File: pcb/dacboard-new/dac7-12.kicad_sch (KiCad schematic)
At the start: 30 parts, among them U22 AD8676xR, U23 AD8676xR, U24 AD8676xR, U25 AD8676xR, U26 AD5791BRUZ, U27 AD5791BRUZ, U28 AD5791BRUZ, U29 AD5791BRUZ, U30 AD8676xR, U31 AD8676xR, U32 AD5791BRUZ, U33 AD5791BRUZ

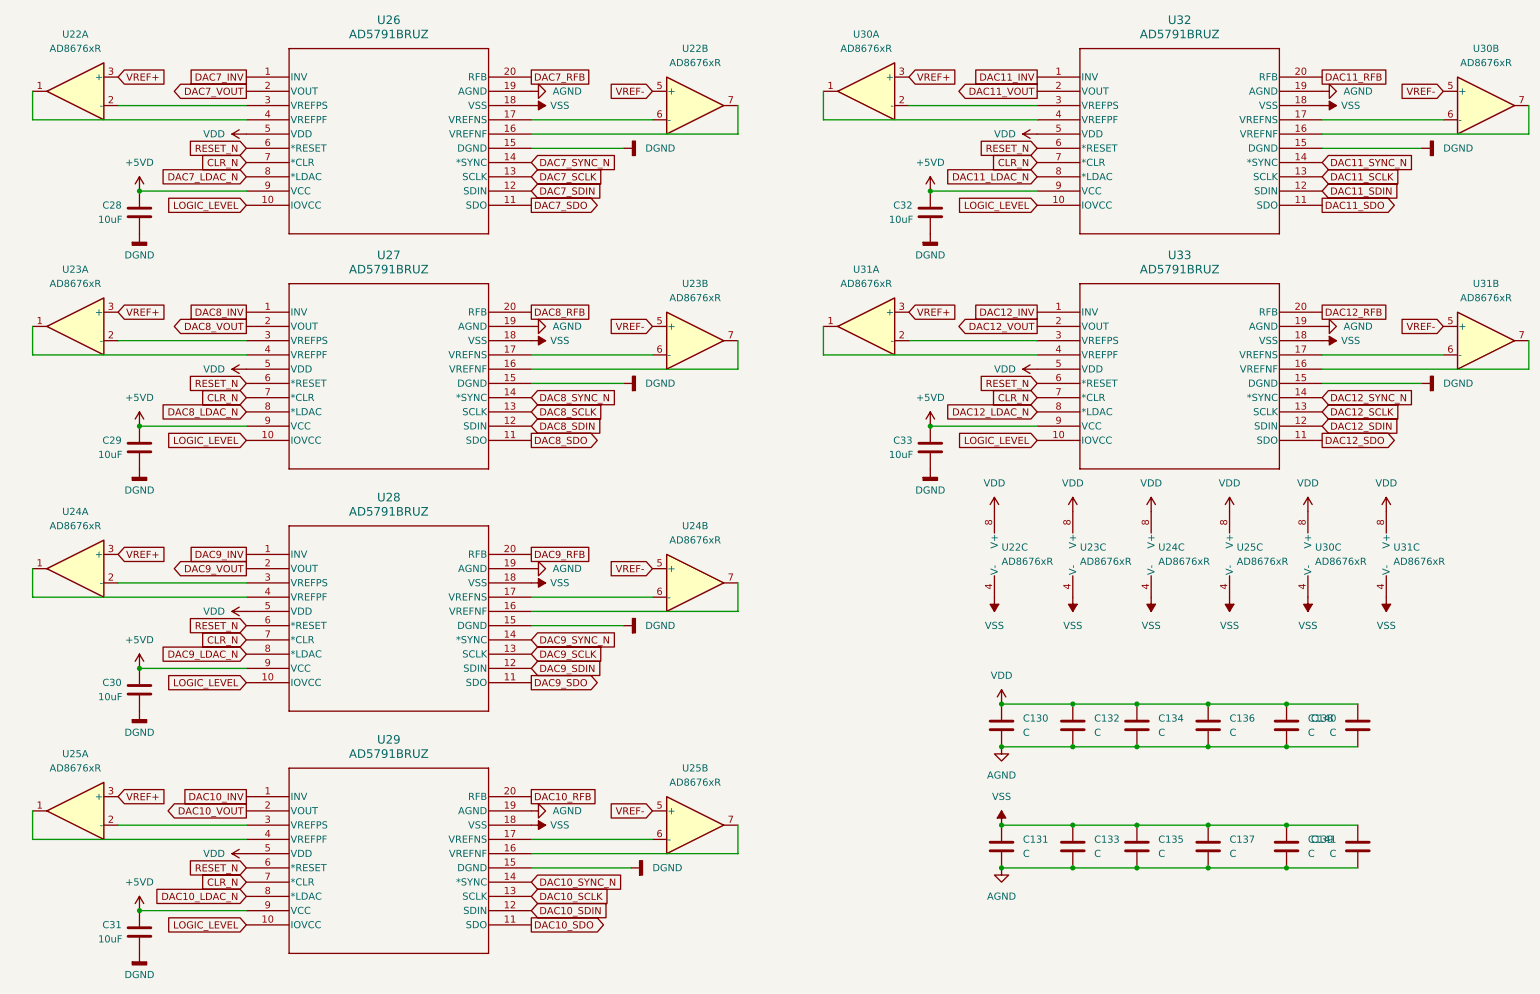
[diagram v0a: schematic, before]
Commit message: new pcb progress
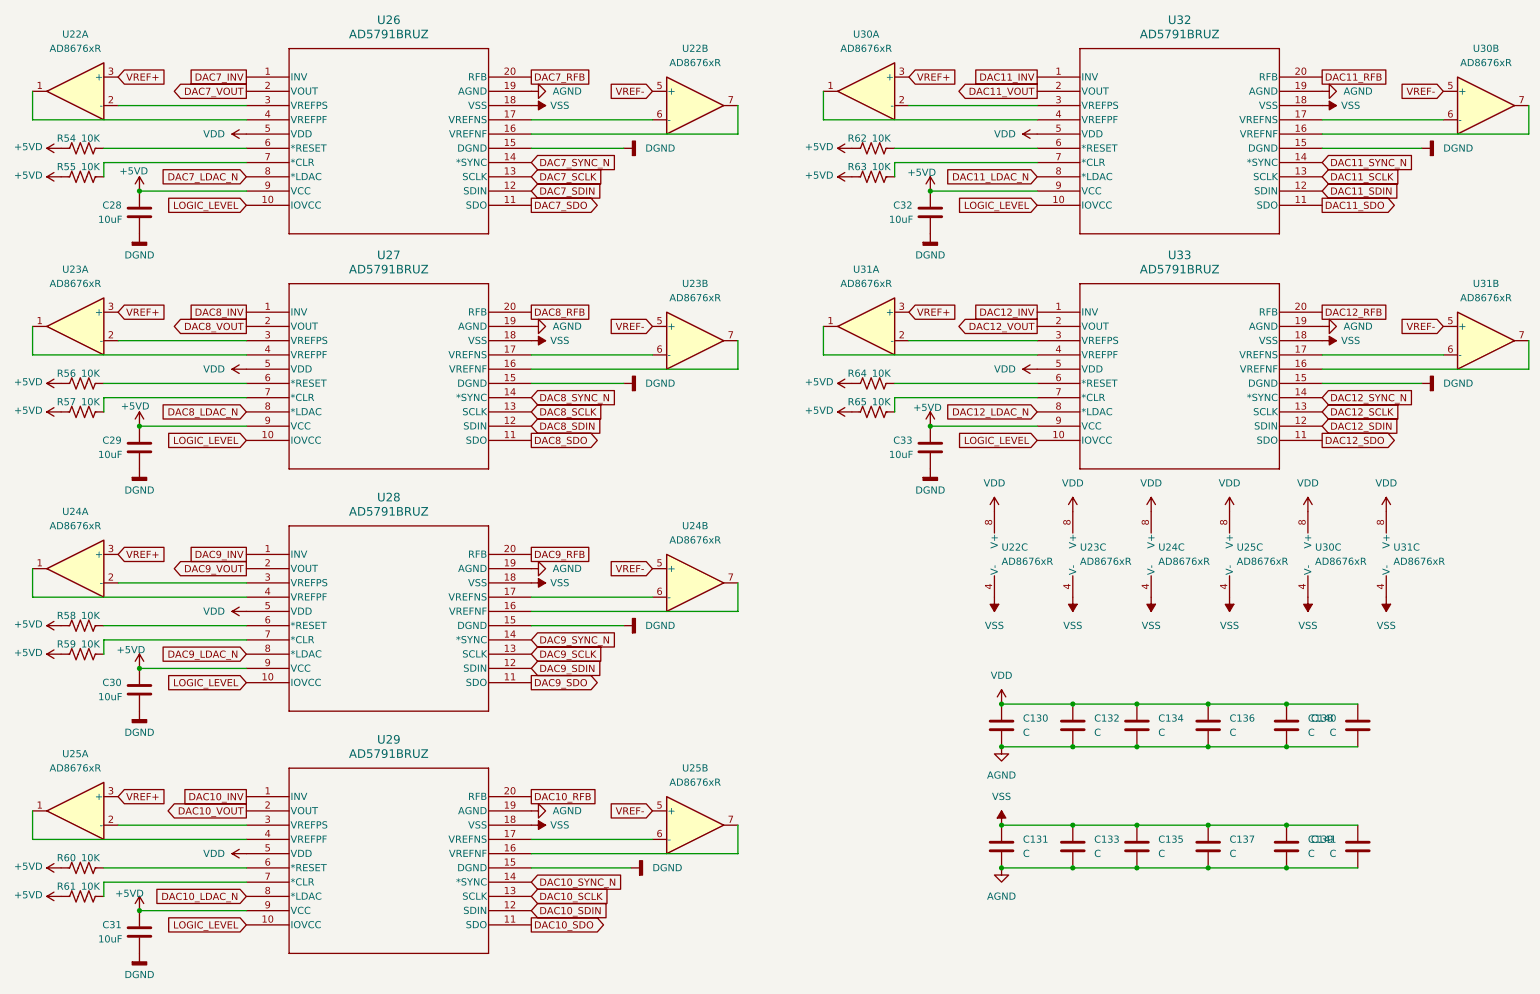
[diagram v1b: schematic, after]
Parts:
- added R54, R55, R56, R57, R58, R59, R60, R61, R62, R63, R64, R65: 10K, Resistor_SMD:R_0402_1005Metric_Pad0.72x0.64mm_HandSolder, symbol Device:R_US
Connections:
- net +5VD: now also R54.1, R55.1, R56.1, R57.1, R58.1, R59.1, R60.1, R61.1, R62.1, R63.1, R64.1, R65.1
- removed net CLR_N: U26.7 (*CLR), U27.7 (*CLR), U28.7 (*CLR), U29.7 (*CLR), U32.7 (*CLR), U33.7 (*CLR)
- removed net RESET_N: U26.6 (*RESET), U27.6 (*RESET), U28.6 (*RESET), U29.6 (*RESET), U32.6 (*RESET), U33.6 (*RESET)
- new net: R64.2, U33.6 (*RESET)
- new net: R54.2, U26.6 (*RESET)
- new net: R55.2, U26.7 (*CLR)
- new net: R62.2, U32.6 (*RESET)
- new net: R63.2, U32.7 (*CLR)
- new net: R58.2, U28.6 (*RESET)
- new net: R60.2, U29.6 (*RESET)
- new net: R65.2, U33.7 (*CLR)
- new net: R61.2, U29.7 (*CLR)
- new net: R59.2, U28.7 (*CLR)
- new net: R56.2, U27.6 (*RESET)
- new net: R57.2, U27.7 (*CLR)
